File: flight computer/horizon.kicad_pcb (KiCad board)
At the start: 4 copper layers, 50.8 x 95.7 mm, 151 parts, among them J1 Micro_SD_Card_Det1, J10 Conn_01x02_Pin, J11 USB_C_Receptacle_USB2.0_16P, J12 Conn_01x04, J13 1x3 servo, J14 1x3 servo, J15 arming terminal, J16 arming terminal, J17 H9161TR-ND, J18 Conn_02x03_Counter_Clockwise, J19 Screw_Terminal_01x02, J20 Screw_Terminal_01x02, J21 Conn_02x03_Counter_Clockwise, J3 H9161TR-ND, J4 H9161TR-ND, J5 Screw_Term, J6 1x3 servo, J9 1x3 servo, Q2 DMG2301L, Q7 BSS138, Q8 IRLML6402, Q9 IRLML6402, SW1 CK_KMS2xxG, U1 MMCU, U10 LSM6DS3, U11 BGM220SC12WGA2R, U13 LTC4412xS6, U15 AP2112K-3.3, U16 SX1262IMLTRT, U17 PE4259, U2 MKL02Z32VFG4, U3 TPS61200DRC, U5 LPS22HB, U6 GPS, U8 NAND, U9 TPS82130, Y1 Crystal, Y2 32MHz

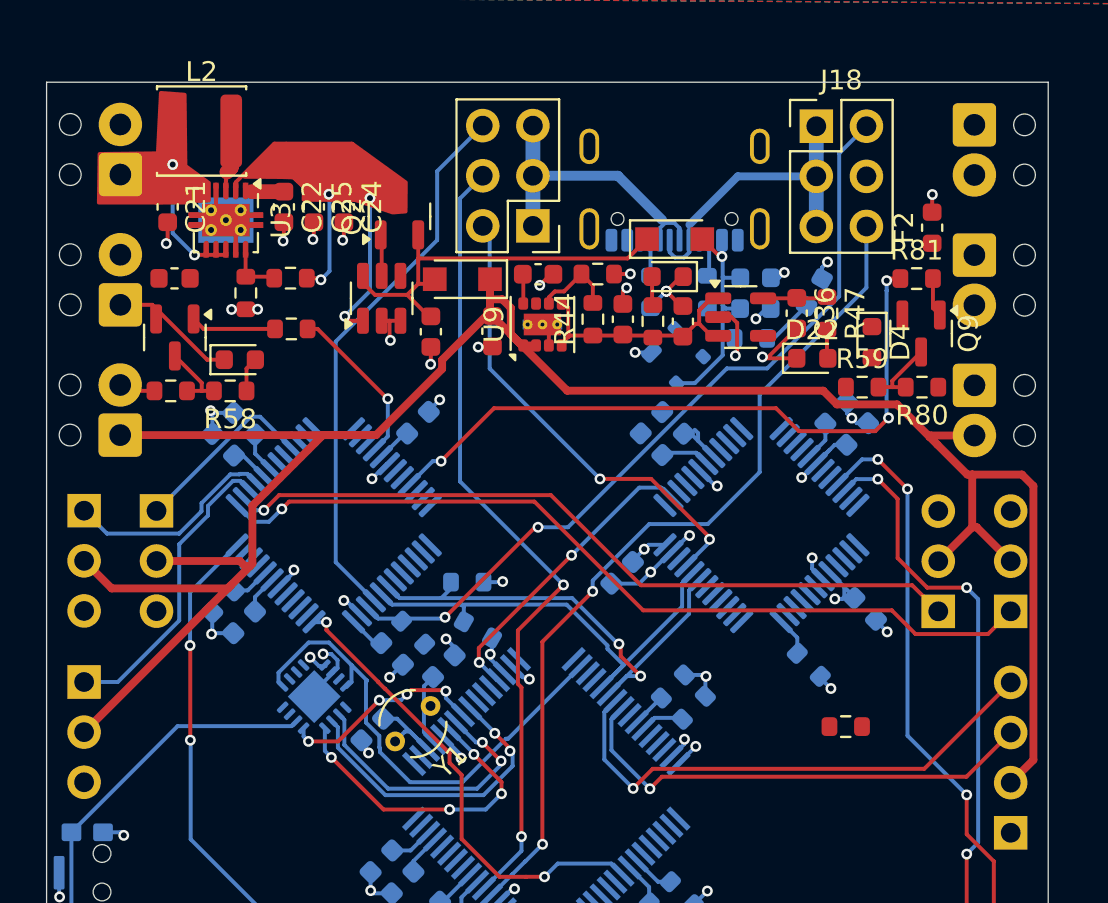
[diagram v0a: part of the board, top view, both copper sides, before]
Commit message: more stuff
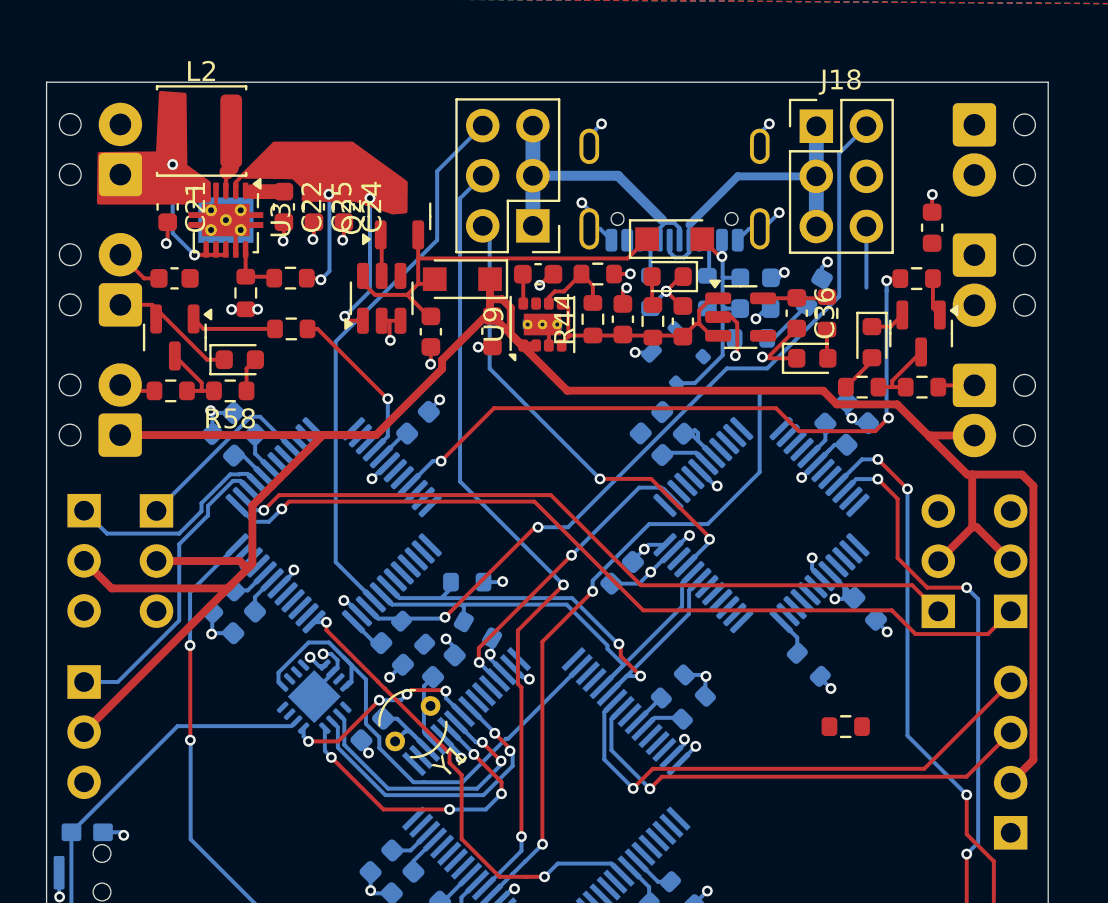
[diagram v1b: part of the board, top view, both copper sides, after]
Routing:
- net GND: track 101.1 -> 109.3 mm, vias 71 -> 75
- net D+ MMCU: track 43.5 -> 35.9 mm
- net Net-(J19-Pin_2): track 0.00 -> 2.45 mm
- net Net-(D4-A): track 0.00 -> 2.04 mm
- net Net-(J16-Pin_1): track 0.00 -> 1.87 mm
- net Net-(D4-K): track 0.00 -> 1.78 mm
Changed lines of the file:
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@@
 			(at 0 -1.43 0)
 			(layer "F.SilkS")
+			(hide yes)
 			(effects
 				(font
@@
 			(at 0 -1.43 0)
 			(layer "F.SilkS")
+			(hide yes)
 			(effects
 				(font
@@
 			(at 0 -1.43 90)
 			(layer "F.SilkS")
+			(hide yes)
 			(effects
 				(font
@@
 			(at 0 -2.4 90)
 			(layer "F.SilkS")
+			(hide yes)
 			(effects
 				(font
@@
 			(at 0 -1.43 0)
 			(layer "F.SilkS")
+			(hide yes)
 			(effects
 				(font
@@
 			(at 0 -1.43 90)
 			(layer "F.SilkS")
+			(hide yes)
 			(effects
 				(font
@@
 			(at 0 -1.43 0)
 			(layer "F.SilkS")
+			(hide yes)
 			(effects
 				(font
@@
 			(at 0 -1.43 90)
 			(layer "F.SilkS")
+			(hide yes)
 			(effects
 				(font
@@
 			(at 0 1.43 0)
 			(layer "B.SilkS")
+			(hide yes)
 			(effects
 				(font
@@
 			(at -0.000001 1.43 60)
 			(layer "B.SilkS")
+			(hide yes)
 			(effects
 				(font
@@
 			(at 0 1.43 45)
 			(layer "B.SilkS")
+			(hide yes)
 			(effects
 				(font
@@
 	)
 	(via
+		(at 195 29)
+		(size 0.55)
+		(drill 0.3)
+		(layers "F.Cu" "B.Cu")
+		(net 1)
+	)
+	(via
 		(at 199.28 33.48)
 		(size 0.55)
@@
 	)
 	(via
+		(at 205 29.5)
+		(size 0.55)
+		(drill 0.3)
+		(layers "F.Cu" "B.Cu")
+		(net 1)
+	)
+	(via
 		(at 205 83)
 		(size 0.55)
@@
 	)
 	(via
+		(at 204.5 25)
+		(size 0.55)
+		(drill 0.3)
+		(layers "F.Cu" "B.Cu")
+		(net 1)
+	)
+	(via
 		(at 197.46 32.6)
 		(size 0.55)
@@
 	)
 	(via
+		(at 196 25)
+		(size 0.55)
+		(drill 0.3)
+		(layers "F.Cu" "B.Cu")
+		(net 1)
+	)
+	(via
 		(at 182.94 49.15)
 		(size 0.55)
@@
 	)
 	(segment
+		(start 195.38 30.32)
+		(end 195.925 30.32)
+		(width 0.2)
+		(layer "B.Cu")
+		(net 1)
+	)
+	(segment
 		(start 188.12 51.1)
 		(end 188.558008 51.538008)
@@
 	)
 	(segment
+		(start 195.38 25.62)
+		(end 196 25)
+		(width 0.2)
+		(layer "B.Cu")
+		(net 1)
+	)
+	(segment
 		(start 186.766016 66.576016)
 		(end 186.7 66.51)
@@
 	)
 	(segment
+		(start 195.38 26.14)
+		(end 195.38 25.62)
+		(width 0.2)
+		(layer "B.Cu")
+		(net 1)
+	)
+	(segment
 		(start 184.193078 56.873079)
 		(end 183.833984 56.513984)
@@
 	)
 	(segment
+		(start 204.02 26.14)
+		(end 204.02 25.48)
+		(width 0.2)
+		(layer "B.Cu")
+		(net 1)
+	)
+	(segment
 		(start 176.273984 49.736016)
 		(end 176.273984 50.816016)
@@
 	)
 	(segment
+		(start 203.475 30.32)
+		(end 202.9 30.895)
+		(width 0.2)
+		(layer "B.Cu")
+		(net 1)
+	)
+	(segment
 		(start 192.019258 53.041367)
 		(end 192.247351 53.041367)
@@
 	)
 	(segment
+		(start 195.925 30.32)
+		(end 196.5 30.895)
+		(width 0.2)
+		(layer "B.Cu")
+		(net 1)
+	)
+	(segment
 		(start 201.766446 43.35)
 		(end 201.86 43.35)
@@
 	)
 	(segment
+		(start 204.02 30.32)
+		(end 203.475 30.32)
+		(width 0.2)
+		(layer "B.Cu")
+		(net 1)
+	)
+	(segment
 		(start 206.67 47.546446)
 		(end 206.67 46.99)
@@
 	)
 	(segment
+		(start 204.02 30.32)
+		(end 204.18 30.32)
+		(width 0.2)
+		(layer "B.Cu")
+		(net 1)
+	)
+	(segment
 		(start 168.515 64.145)
 		(end 168.54 64.17)
@@
 	)
 	(segment
+		(start 204.02 25.48)
+		(end 204.5 25)
+		(width 0.2)
+		(layer "B.Cu")
+		(net 1)
+	)
+	(segment
 		(start 204.57 34.36)
 		(end 204.34 34.36)
@@
 	)
 	(segment
+		(start 195.38 29.38)
+		(end 195 29)
+		(width 0.2)
+		(layer "B.Cu")
+		(net 1)
+	)
+	(segment
 		(start 200.2 56.417891)
 		(end 200.2 56.18)
@@
 	)
 	(segment
+		(start 195.38 30.32)
+		(end 195.38 29.38)
+		(width 0.2)
+		(layer "B.Cu")
+		(net 1)
+	)
+	(segment
 		(start 182.372722 52.831973)
 		(end 181.48 53.724695)
@@
 	)
 	(segment
+		(start 204.18 30.32)
+		(end 205 29.5)
+		(width 0.2)
+		(layer "B.Cu")
+		(net 1)
+	)
+	(segment
 		(start 170.74 60.895)
 		(end 171.635 60.895)
@@
 	)
 	(segment
+		(start 208.413372 48.582712)
+		(end 208.413372 48.892105)
+		(width 0.2)
+		(layer "B.Cu")
+		(net 2)
+	)
+	(segment
+		(start 208.30033 48.46967)
+		(end 208.413372 48.582712)
+		(width 0.2)
+		(layer "B.Cu")
+		(net 2)
+	)
+	(segment
 		(start 200.89033 40.66967)
 		(end 200.89033 41.05967)
@@
 	)
 	(segment
+		(start 209.7 35.275)
+		(end 210.65 35.275)
+		(width 0.2)
+		(layer "F.Cu")
+		(net 11)
+	)
+	(segment
+		(start 210.65 35.275)
+		(end 211.24 34.685)
+		(width 0.2)
+		(layer "F.Cu")
+		(net 11)
+	)
+	(segment
+		(start 172.82 32.83)
+		(end 173.575 32.83)
+		(width 0.2)
+		(layer "F.Cu")
+		(net 13)
+	)
+	(segment
+		(start 171.62 31.63)
+		(end 172.82 32.83)
+		(width 0.2)
+		(layer "F.Cu")
+		(net 13)
+	)
+	(segment
 		(start 177.325979 43.088697)
 		(end 176.058 44.356676)
@@
 	)
 	(segment
-		(start 184.774078 56.63242)
-		(end 184.774078 56.834078)
+		(start 184.063716 55.403672)
+		(end 184.739 56.078956)
 		(width 0.2)
 		(layer "B.Cu")
@@
 	)
 	(segment
-		(start 184.739 56.011076)
-		(end 184.739 56.597342)
+		(start 182.953794 52.046206)
+		(end 184.063716 53.156128)
 		(width 0.2)
 		(layer "B.Cu")
@@
 	(segment
 		(start 182.186589 51.279)
-		(end 183.329649 52.42206)
+		(end 182.953794 52.046206)
 		(width 0.2)
 		(layer "B.Cu")
@@
 	)
 	(segment
-		(start 184.739 56.597342)
-		(end 184.774078 56.63242)
+		(start 184.739 56.621786)
+		(end 186.474893 58.357679)
 		(width 0.2)
 		(layer "B.Cu")
@@
 	)
 	(segment
-		(start 184.774078 56.834078)
-		(end 186.297679 58.357679)
+		(start 184.739 56.078956)
+		(end 184.739 56.621786)
 		(width 0.2)
 		(layer "B.Cu")
@@
 	)
 	(segment
-		(start 186.297679 58.357679)
+		(start 187 58.357679)
 		(end 188.952321 58.357679)
 		(width 0.2)
@@
 	)
 	(segment
-		(start 184.063716 55.335792)
-		(end 184.739 56.011076)
-		(width 0.2)
-		(layer "B.Cu")
-		(net 22)
-	)
-	(segment
 		(start 188.952321 58.357679)
 		(end 191.155 56.155)
@@
 	)
 	(segment
-		(start 184.063716 53.268695)
-		(end 184.063716 55.335792)
+		(start 184.063716 53.156128)
+		(end 184.063716 55.403672)
 		(width 0.2)
 		(layer "B.Cu")
@@
 	)
 	(segment
-		(start 183.329649 52.42206)
-		(end 184.12 53.212411)
+		(start 179.630351 53.28926)
+		(end 179.630351 52.805398)
 		(width 0.2)
 		(layer "B.Cu")
@@
 	)
 	(segment
-		(start 179.630351 53.28926)
-		(end 179.630351 52.805398)
+		(start 186.474893 58.357679)
+		(end 187 58.357679)
 		(width 0.2)
 		(layer "B.Cu")
@@
 	)
 	(segment
-		(start 184.12 53.212411)
-		(end 184.063716 53.268695)
+		(start 182.953794 52.046206)
+		(end 183.329649 52.42206)
 		(width 0.2)
 		(layer "B.Cu")
@@
 	)
 	(segment
-		(start 209.42 33.3)
-		(end 204.01 38.71)
-		(width 0.2)
-		(layer "B.Cu")
-		(net 27)
-	)
-	(segment
 		(start 191.491449 63.008551)
 		(end 191.49 63.008551)
@@
 	)
 	(segment
+		(start 213.15 38.25)
+		(end 213.06 38.34)
+		(width 0.2)
+		(layer "F.Cu")
+		(net 154)
+	)
+	(segment
+		(start 214.8925 38.25)
+		(end 213.15 38.25)
+		(width 0.2)
+		(layer "F.Cu")
+		(net 154)
+	)
+	(segment
 		(start 176.96406 31.639289)
 		(end 175.96406 31.639289)
@@
 	)
 	(segment
+		(start 209.7 37.02)
+		(end 208.38 38.34)
+		(width 0.2)
+		(layer "F.Cu")
+		(net 161)
+	)
+	(segment
+		(start 209.7 36.85)
+		(end 209.7 37.02)
+		(width 0.2)
+		(layer "F.Cu")
+		(net 161)
+	)
+	(segment
